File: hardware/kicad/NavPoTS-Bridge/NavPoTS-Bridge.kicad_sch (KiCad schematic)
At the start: 74 parts, among them J1 Conn_01x06_Pin, J2 USB_C_Receptacle_USB2.0_16P, J3 Screw_Terminal_01x06, J4 Conn_02x04_Top_Bottom, J5 Conn_02x04_Top_Bottom, J6 Conn_02x04_Top_Bottom, J7 62684-402100ALF, J8 62684-402100ALF, J9 Conn_02x04_Top_Bottom, U1 MS5611-01BA, U2 H3LIS331DLTR, U3 ASM330LHHXTR, U4 MMC5983MA, U5 USBLC6-2SC6, U6 STM32H743ZITx, Y1 ECS-2520MV-xxx-xx

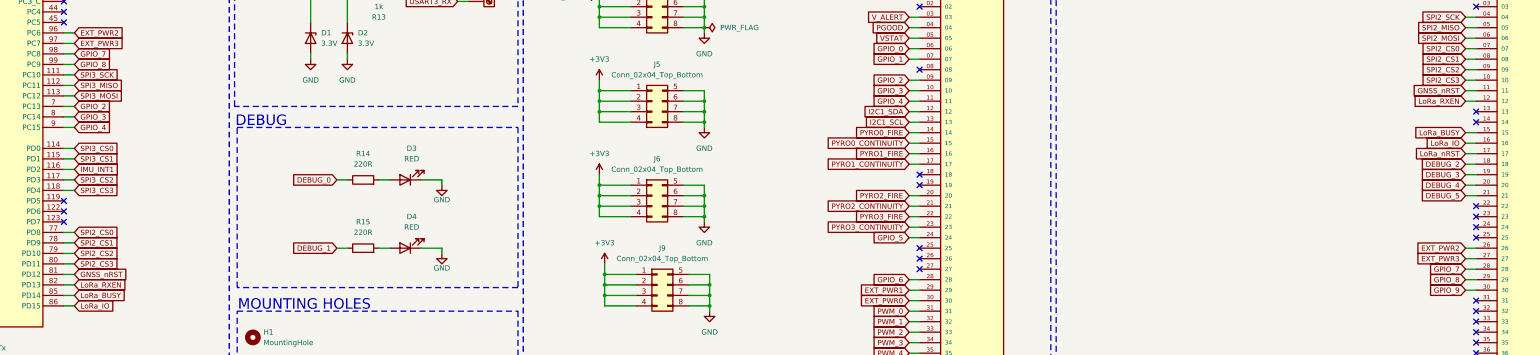
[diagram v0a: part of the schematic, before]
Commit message: v1.0
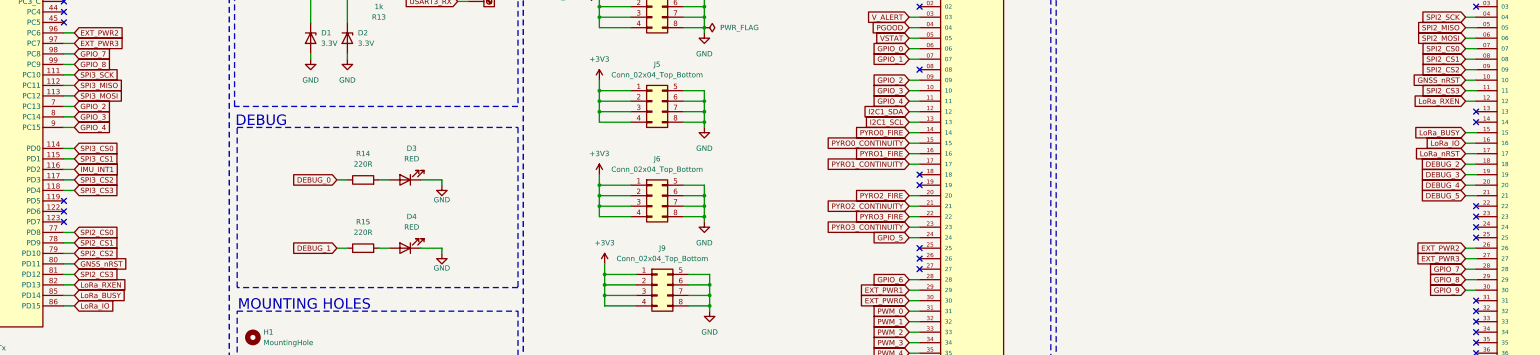
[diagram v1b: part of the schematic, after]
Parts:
- J4, J5, J6, J9: MPN (none) -> PEC14SAGN; Manufacturer (none) -> Sullins Connector Solutions
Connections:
- net GNSS_nRST: now also J7.10, U6.80 (PD11); no longer J7.11, U6.81 (PD12)
- net SPI2_CS3: now also J7.11, U6.81 (PD12); no longer J7.10, U6.80 (PD11)
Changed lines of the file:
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@@
 	(global_label "SPI2_CS3"
 		(shape input)
-		(at 200.66 237.49 0)
+		(at 200.66 240.03 0)
 		(fields_autoplaced yes)
 		(effects
@@
 		)
 		(property "Intersheetrefs" "${INTERSHEET_REFS}"
-			(at 212.5956 237.49 0)
+			(at 212.5956 240.03 0)
 			(effects
 				(font
@@
 	(global_label "SPI2_CS3"
 		(shape input)
-		(at 537.21 193.04 180)
+		(at 537.21 195.58 180)
 		(fields_autoplaced yes)
 		(effects
@@
 		)
 		(property "Intersheetrefs" "${INTERSHEET_REFS}"
-			(at 525.2744 193.04 0)
+			(at 525.2744 195.58 0)
 			(effects
 				(font
@@
 	(global_label "GNSS_nRST"
 		(shape input)
-		(at 537.21 195.58 180)
+		(at 537.21 193.04 180)
 		(fields_autoplaced yes)
 		(effects
@@
 		)
 		(property "Intersheetrefs" "${INTERSHEET_REFS}"
-			(at 523.6416 195.58 0)
+			(at 523.6416 193.04 0)
 			(effects
 				(font
@@
 	(global_label "GNSS_nRST"
 		(shape input)
-		(at 200.66 240.03 0)
+		(at 200.66 237.49 0)
 		(fields_autoplaced yes)
 		(effects
@@
 		)
 		(property "Intersheetrefs" "${INTERSHEET_REFS}"
-			(at 214.2284 240.03 0)
+			(at 214.2284 237.49 0)
 			(effects
 				(font
@@
 			)
 		)
+		(property "MPN" "PEC14SAGN"
+			(at 340.36 198.12 0)
+			(effects
+				(font
+					(size 1.27 1.27)
+				)
+				(hide yes)
+			)
+		)
+		(property "Manufacturer" "Sullins Connector Solutions"
+			(at 340.36 198.12 0)
+			(effects
+				(font
+					(size 1.27 1.27)
+				)
+				(hide yes)
+			)
+		)
 		(pin "6"
 		)
@@
 			)
 		)
+		(property "MPN" "PEC14SAGN"
+			(at 341.63 242.57 0)
+			(effects
+				(font
+					(size 1.27 1.27)
+				)
+				(hide yes)
+			)
+		)
+		(property "Manufacturer" "Sullins Connector Solutions"
+			(at 341.63 242.57 0)
+			(effects
+				(font
+					(size 1.27 1.27)
+				)
+				(hide yes)
+			)
+		)
 		(pin "6"
 		)
@@
 			)
 		)
+		(property "MPN" "PEC14SAGN"
+			(at 340.36 175.26 0)
+			(effects
+				(font
+					(size 1.27 1.27)
+				)
+				(hide yes)
+			)
+		)
+		(property "Manufacturer" "Sullins Connector Solutions"
+			(at 340.36 175.26 0)
+			(effects
+				(font
+					(size 1.27 1.27)
+				)
+				(hide yes)
+			)
+		)
 		(pin "6"
 		)
@@
 			(at 340.36 220.98 0)
 			(effects
+				(font
+					(size 1.27 1.27)
+				)
+				(hide yes)
+			)
+		)
+		(property "MPN" "PEC14SAGN"
+			(at 340.36 220.98 0)
+			(effects
+				(font
+					(size 1.27 1.27)
+				)
+				(hide yes)
+			)
+		)
+		(property "Manufacturer" "Sullins Connector Solutions"
+			(at 340.36 220.98 0)
+			(effects
